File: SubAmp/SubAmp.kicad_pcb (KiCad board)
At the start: 2 copper layers, 170.4 x 67 mm, 55 parts, among them J1 OUT, J2 VCC, J3 VEE, J4 GND, J6 IN, Q1 MPSA42, Q10 2SA1943, Q11 2SC5200, Q12 2SA1943, Q2 MPSA42, Q3 MPSA42, Q4 MJE15033, Q5 MJE15032, Q6 MJE15033, Q7 2SA1943, Q8 2SC5200, Q9 2SC5200

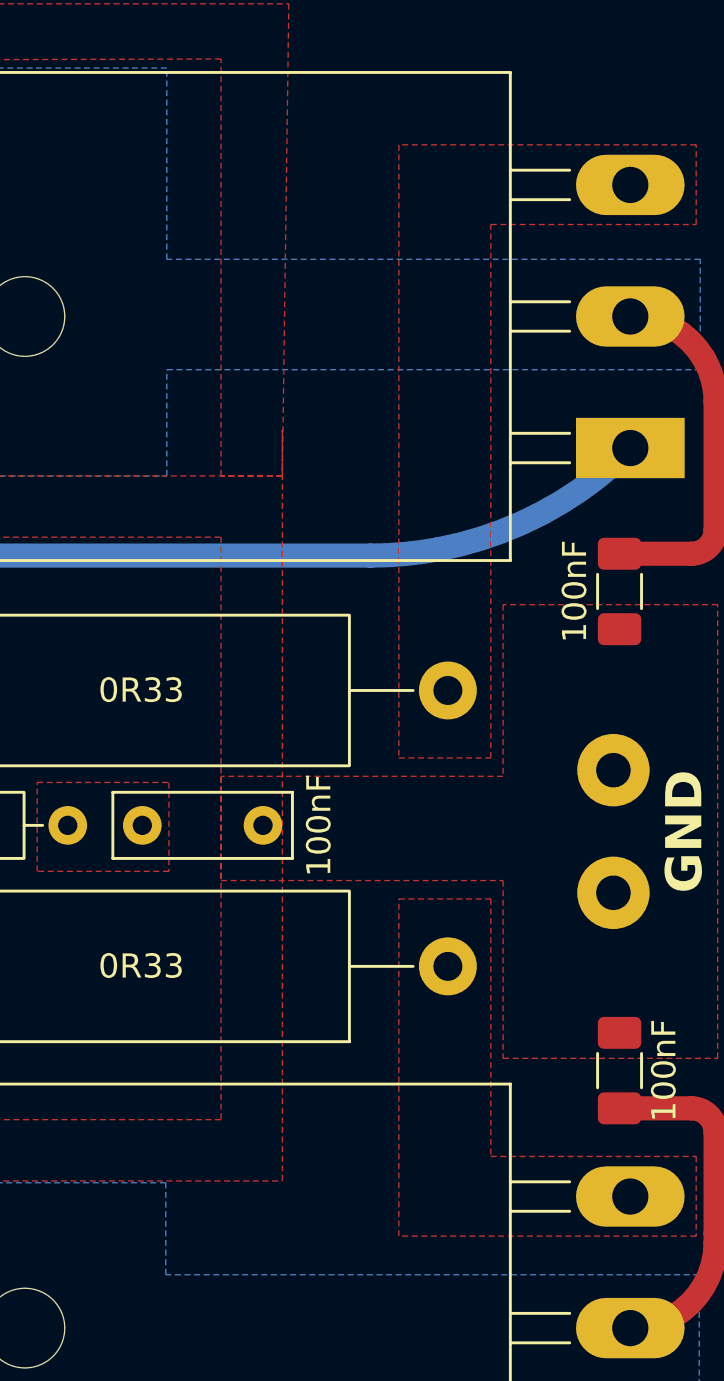
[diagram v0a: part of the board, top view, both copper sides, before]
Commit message: more work
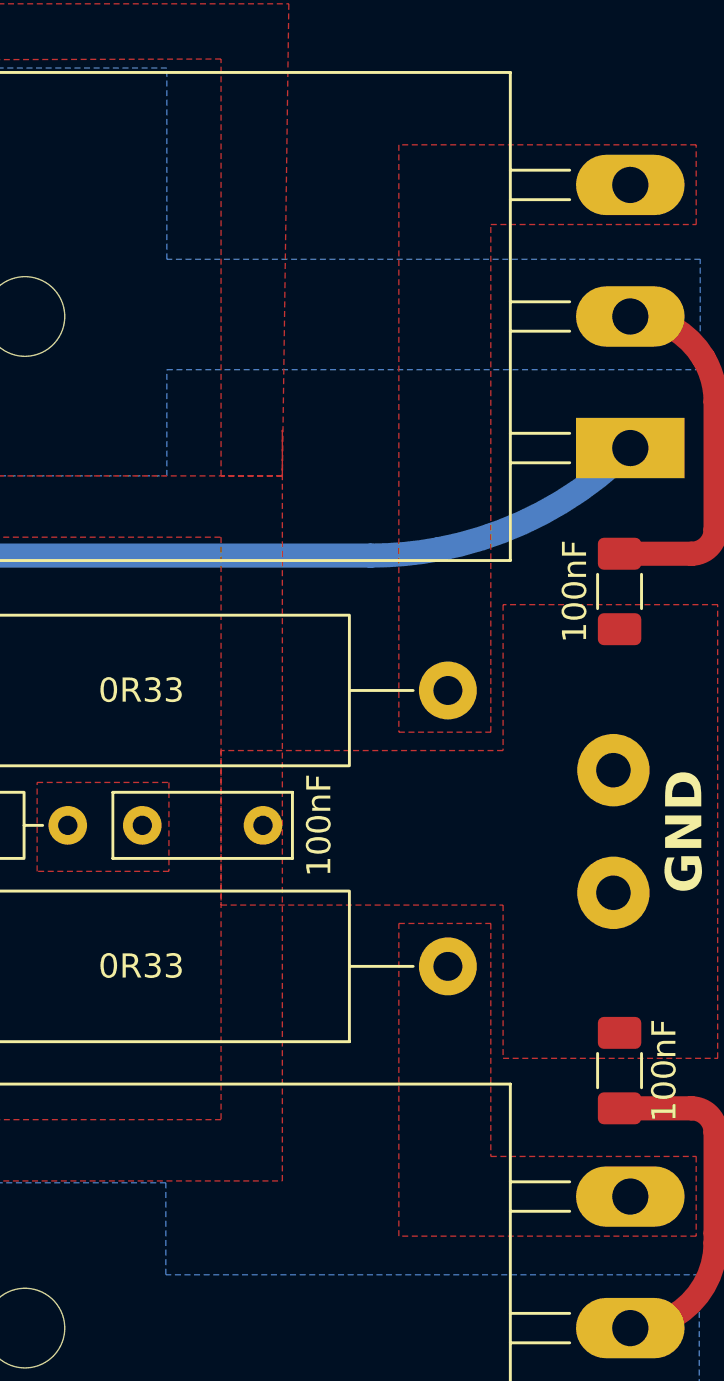
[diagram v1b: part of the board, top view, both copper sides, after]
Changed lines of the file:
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@@
 		(polygon
 			(pts
-				(xy 183.515 82.804) (xy 171.196 82.804) (xy 171.196 108.204) (xy 175.006 108.204) (xy 175.006 86.106)
+				(xy 183.515 82.804) (xy 171.196 82.804) (xy 171.196 107.1372) (xy 175.006 107.1372) (xy 175.006 86.106)
 				(xy 183.515 86.106)
 			)
@@
 		(polygon
 			(pts
-				(xy 183.515 128.016) (xy 171.196 128.016) (xy 171.196 114.046) (xy 175.006 114.046) (xy 175.006 124.714)
+				(xy 183.515 128.016) (xy 171.196 128.016) (xy 171.196 115.062) (xy 175.006 115.062) (xy 175.006 124.714)
 				(xy 183.515 124.714)
 			)
@@
 		(polygon
 			(pts
-				(xy 163.83 108.966) (xy 163.83 113.284) (xy 175.514 113.284) (xy 175.514 120.65) (xy 184.404 120.65)
-				(xy 184.404 101.854) (xy 175.514 101.854) (xy 175.514 108.966)
-			)
-		)
+				(xy 163.83 107.8992) (xy 163.83 114.3) (xy 175.514 114.3) (xy 175.514 120.65) (xy 184.404 120.65)
+				(xy 184.404 101.854) (xy 175.514 101.854) (xy 175.514 107.8992)
+			)
+		)
